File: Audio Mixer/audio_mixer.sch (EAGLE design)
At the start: 33 parts, among them IC2 LM747CN

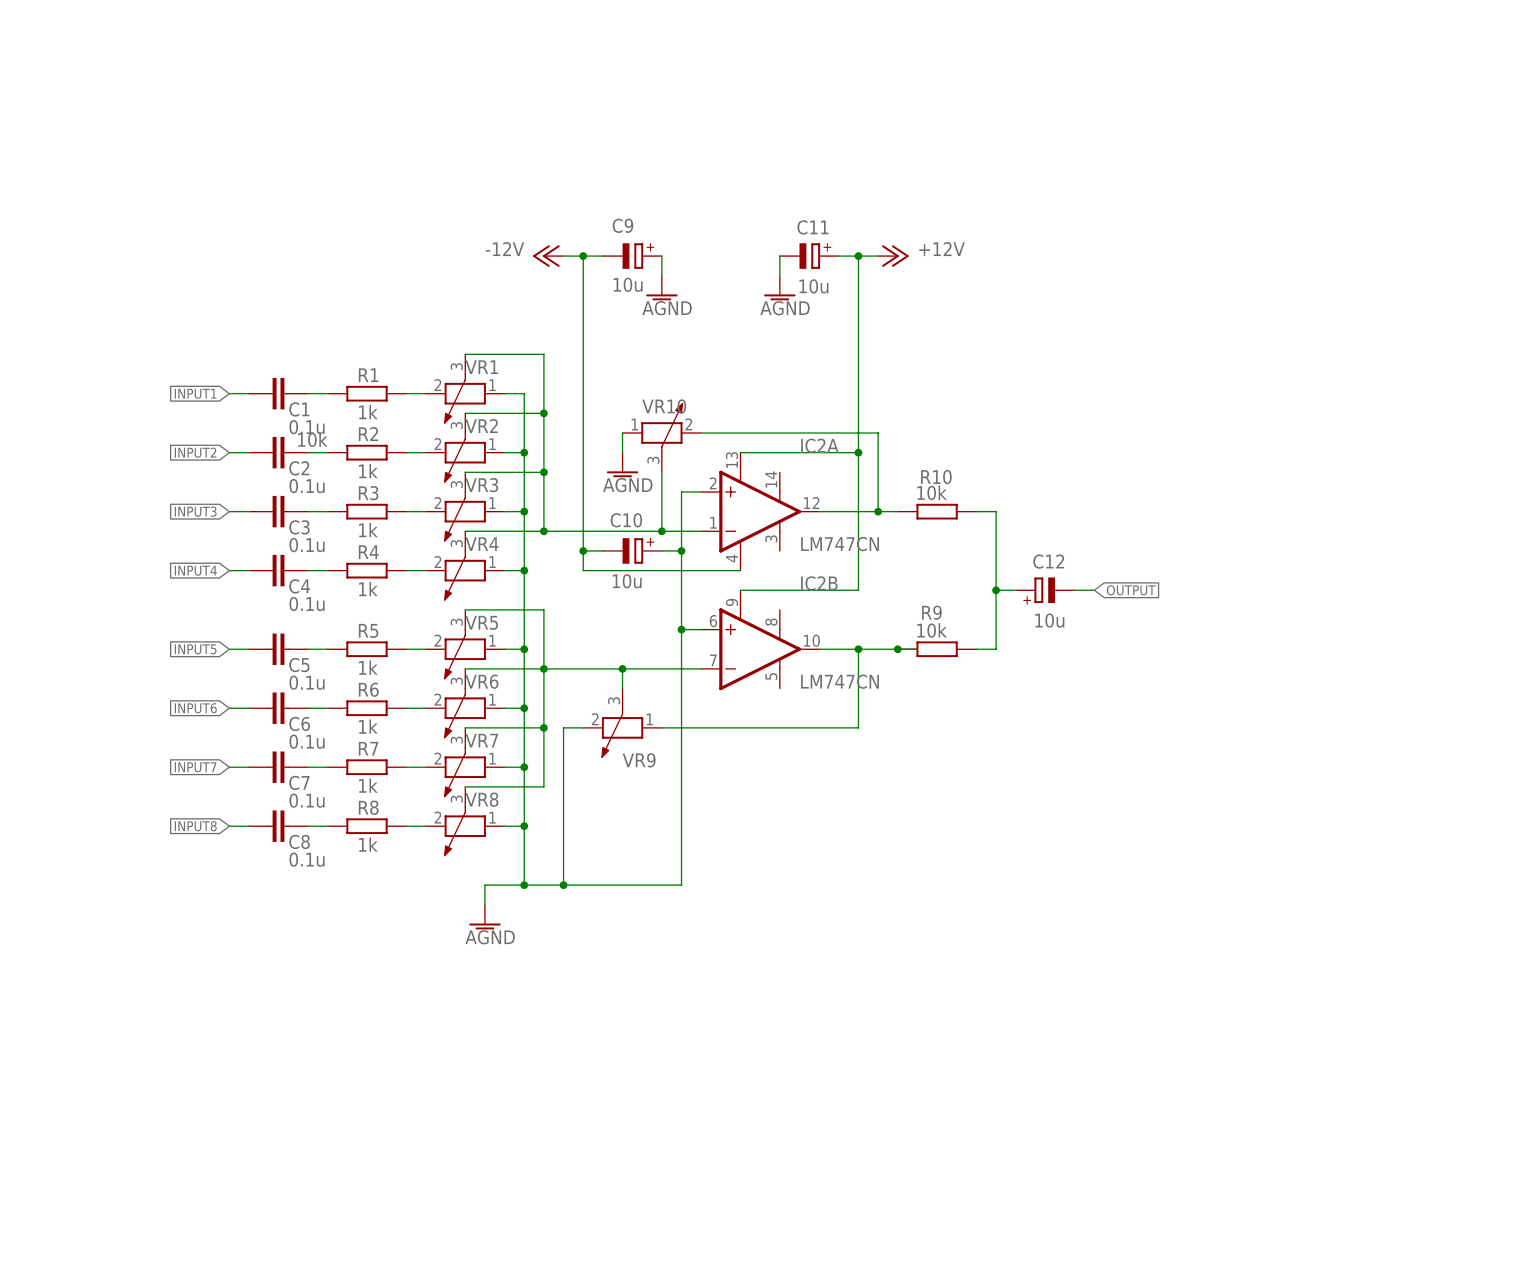
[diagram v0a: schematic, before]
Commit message: Mixer Design complete
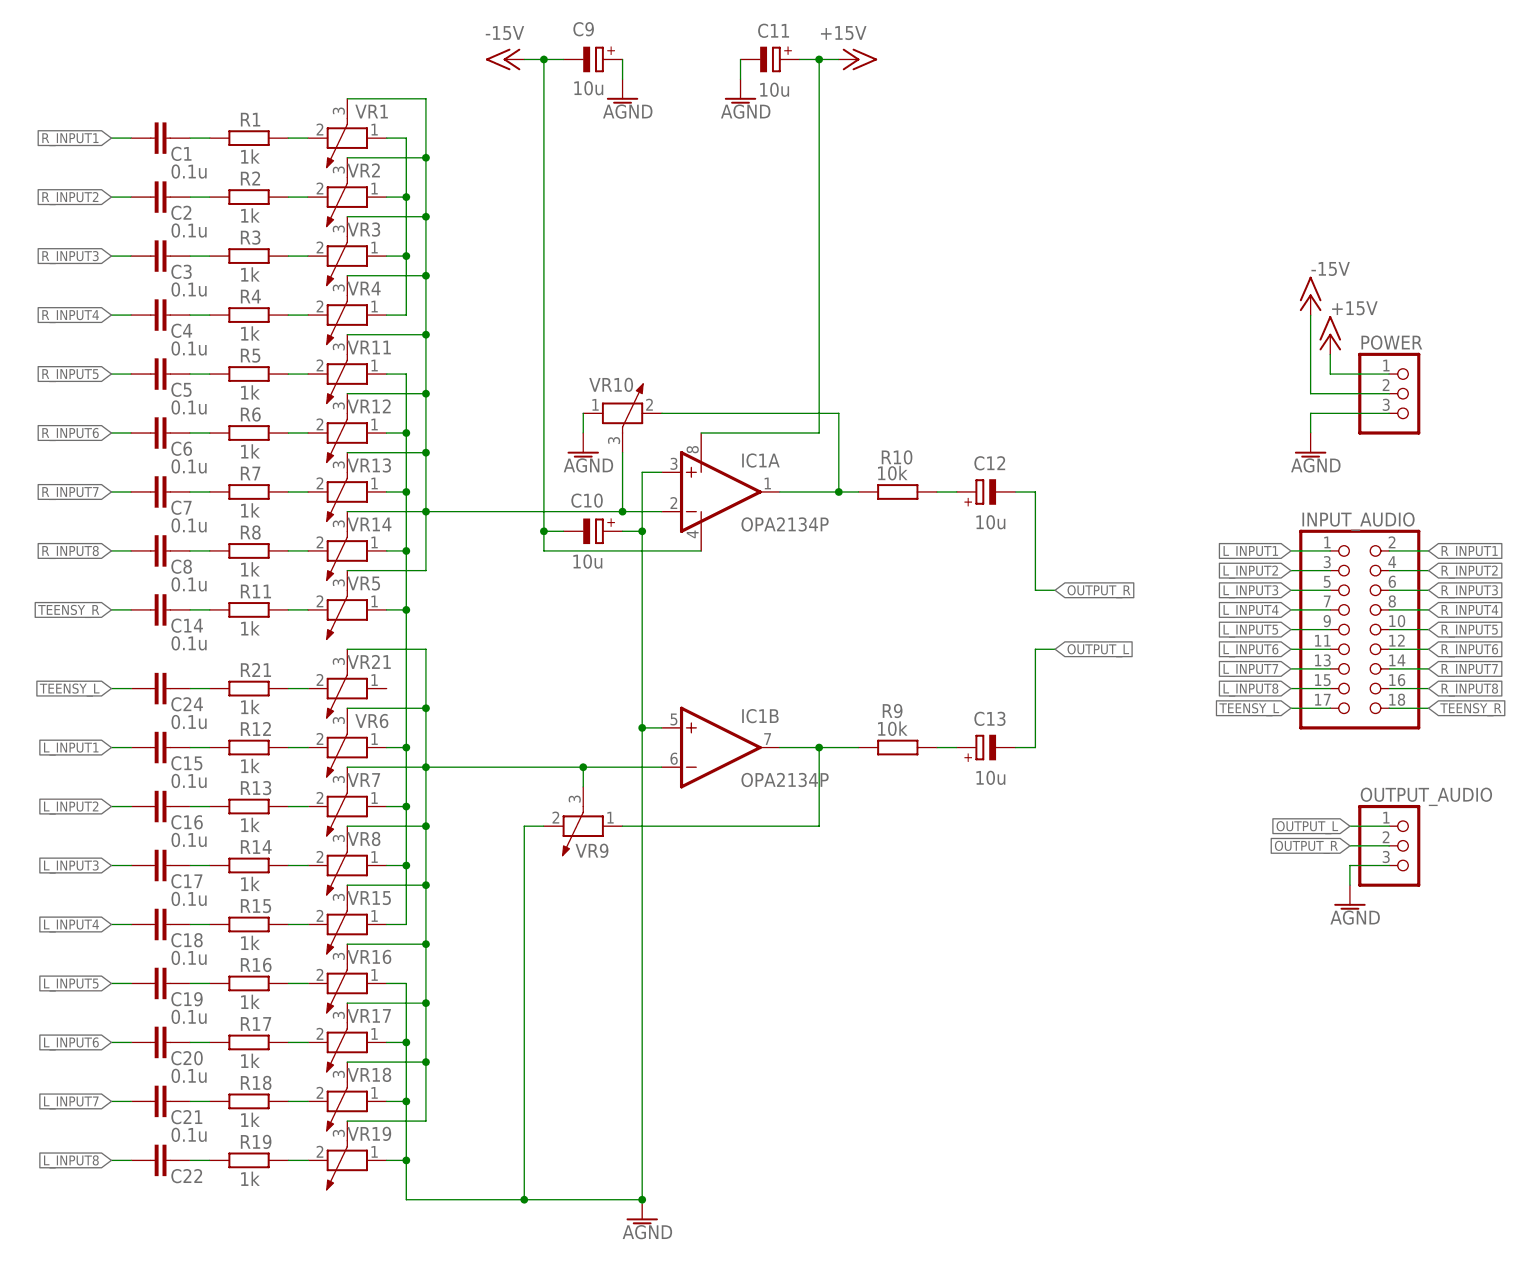
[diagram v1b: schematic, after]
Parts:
- removed IC2: LM747CN, linear:LM747CN
- added C13: 10u, rcl:CPOL-EUE5-10.5
- added C14, C15, C16, C17, C18, C19, C20, C21, C22, C24: 0.1u, rcl:C-EU025-030X050
- added IC1: OPA2134P, linear:OPA2134P
- added INPUT_AUDIO: (no value), pinhead:PINHD-2X9
- added OUTPUT_AUDIO, POWER: (no value), pinhead:PINHD-1X3
- added R11, R12, R13, R14, R15, R16, R17, R18, R19, R21: 1k, rcl:R-EU_R0805
- added VR11, VR16: 10k, rcl:POTENTIOMETER_PT-10
- added VR12, VR13, VR14, VR15, VR17, VR18, VR19, VR21: (no value), rcl:POTENTIOMETER_PT-10
- VR6: value (none) -> 10k
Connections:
- removed net +12V: C11.+, IC2A.V+, IC2B.V+
- removed net -12V: C10.-, C9.-, IC2P.V-
- removed net INPUT1: C1.2
- removed net INPUT2: C2.2
- removed net INPUT3: C3.2
- removed net INPUT4: C4.2
- removed net INPUT5: C5.2
- removed net INPUT6: C6.2
- removed net INPUT7: C7.2
- removed net INPUT8: C8.2
- removed net OUTPUT: C12.-
- new net +15V: C11.+, IC1P.V+, POWER.1
- new net -15V: C10.-, C9.-, IC1P.V-, POWER.2
- new net L_INPUT1: C15.2, INPUT_AUDIO.1
- new net L_INPUT2: C16.2, INPUT_AUDIO.3
- new net L_INPUT3: C17.2, INPUT_AUDIO.5
- new net L_INPUT4: C18.2, INPUT_AUDIO.7
- new net L_INPUT5: C19.2, INPUT_AUDIO.9
- new net L_INPUT6: C20.2, INPUT_AUDIO.11
- new net L_INPUT7: C21.2, INPUT_AUDIO.13
- new net L_INPUT8: C22.2, INPUT_AUDIO.15
- new net N$20: C13.+, R9.1
- new net N$23: R13.2, VR7.2
- new net N$24: VR1.1, VR2.1, VR3.1, VR4.1
- new net N$28: R7.2, VR13.2
- new net N$29: R5.2, VR11.2
- new net N$30: R6.2, VR12.2
- new net N$32: R8.2, VR14.2
- new net N$34: VR11.1, VR12.1, VR13.1, VR14.1, VR15.1, VR5.1, VR6.1, VR7.1, VR8.1
- new net N$35: C18.1, R15.1
- new net N$36: R15.2, VR15.2
- new net N$37: IC1B.-IN, VR15.3, VR16.3, VR17.3, VR18.3, VR19.3, VR21.3, VR6.3, VR7.3, VR8.3, VR9.3
- new net N$39: C19.1, R16.1
- new net N$40: C20.1, R17.1
- new net N$41: C21.1, R18.1
- new net N$42: R18.2, VR18.2
- new net N$43: R16.2, VR16.2
- new net N$44: R17.2, VR17.2
- new net N$45: C22.1, R19.1
- new net N$46: R19.2, VR19.2
- new net N$6: C14.1, R11.1
- new net N$7: R11.2, VR5.2
- new net N$8: C24.1, R21.1
- new net N$9: R21.2, VR21.2
- new net OUTPUT_L: C13.-, OUTPUT_AUDIO.1
- new net OUTPUT_R: C12.-, OUTPUT_AUDIO.2
- new net R_INPUT1: C1.2, INPUT_AUDIO.2
- new net R_INPUT2: C2.2, INPUT_AUDIO.4
- new net R_INPUT3: C3.2, INPUT_AUDIO.6
- new net R_INPUT4: C4.2, INPUT_AUDIO.8
- new net R_INPUT5: C5.2, INPUT_AUDIO.10
- new net R_INPUT6: C6.2, INPUT_AUDIO.12
- new net R_INPUT7: C7.2, INPUT_AUDIO.14
- new net R_INPUT8: C8.2, INPUT_AUDIO.16
- new net TEENSY_L: C24.2, INPUT_AUDIO.17
- new net TEENSY_R: C14.2, INPUT_AUDIO.18
- net AGND: now also IC1A.+IN, IC1B.+IN, OUTPUT_AUDIO.3, POWER.3, VR16.1, VR17.1, VR18.1, VR19.1; no longer IC2A.+IN, IC2B.+IN, VR1.1, VR2.1, VR3.1, VR4.1, VR5.1, VR6.1, VR7.1, VR8.1
- net N$11: now also C15.1, R12.1; no longer IC2B.-IN, VR5.3, VR6.3, VR7.3, VR8.3, VR9.3
- net N$12: now also IC1A.-IN, VR11.3, VR12.3, VR13.3, VR14.3, VR5.3; no longer IC2A.-IN
- net N$15: now also C16.1, R13.1; no longer R5.2, VR5.2
- net N$16: now also C17.1, R14.1; no longer R6.2, VR6.2
- net N$17: now also R14.2, VR8.2; no longer R7.2, VR7.2
- net N$19: now also IC1A.OUT; no longer IC2A.OUT
- net N$2: no longer R9.1
- net N$21: now also R12.2, VR6.2; no longer R8.2, VR8.2
- net N$22: now also IC1B.OUT; no longer IC2B.OUT
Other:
- note added: "Audio inputs. MIC level"
- note added: "LEFT Gain control"
- note added: "Level adj, weight control"
- note added: "RIGHT Gain control"
- note added: "To pre-amp"
- moved on the sheet: C1, C10, C11, C12, C2, C3, C4, C5, C6, C7, C8, C9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
